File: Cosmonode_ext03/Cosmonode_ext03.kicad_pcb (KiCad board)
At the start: 2 copper layers, 23.5 x 34.3 mm, 8 parts, among them J1 CONN_01X04, J2 GS3, J3 GS3, J4 CONN_01X04, J5 CONN_01X08, J6 CONN_01X08, J7 Aloes_Logo, J8 OSHW_Logo

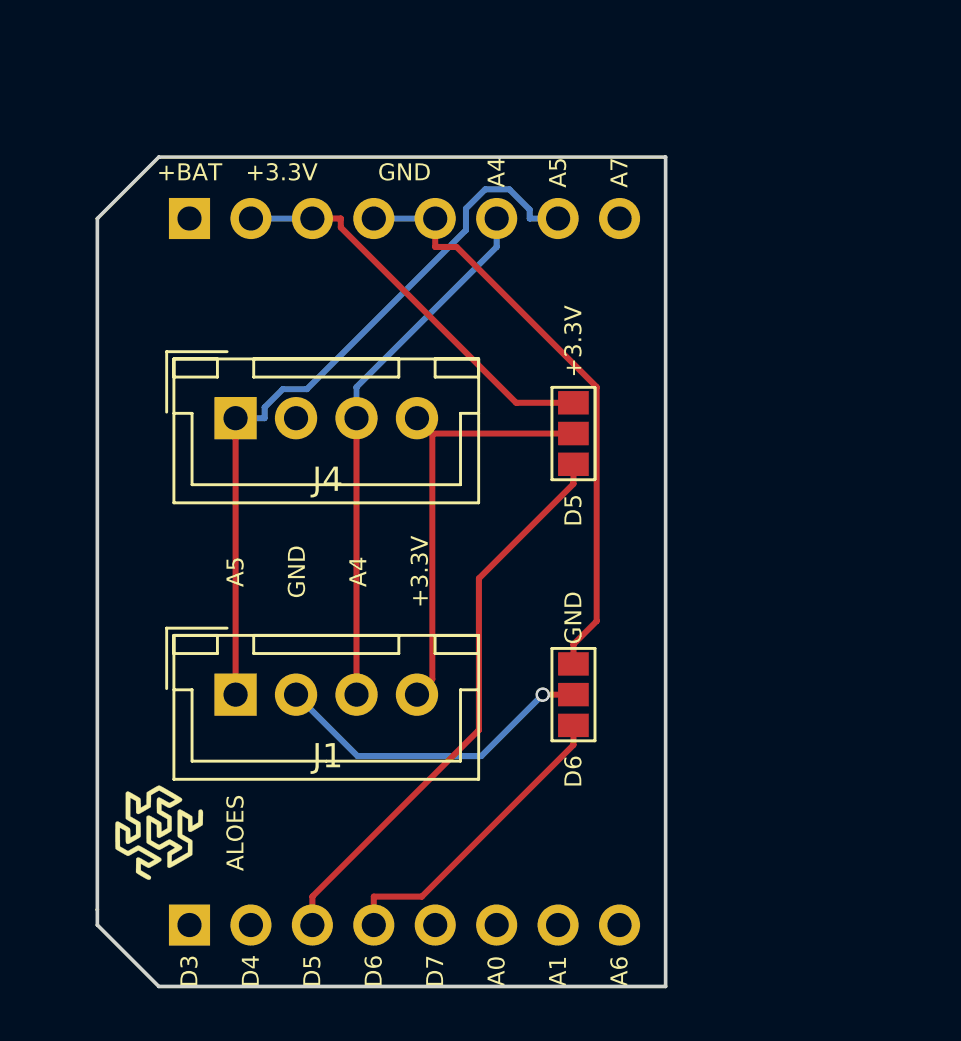
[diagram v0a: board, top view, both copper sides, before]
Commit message: update to V0.7 (WIP)
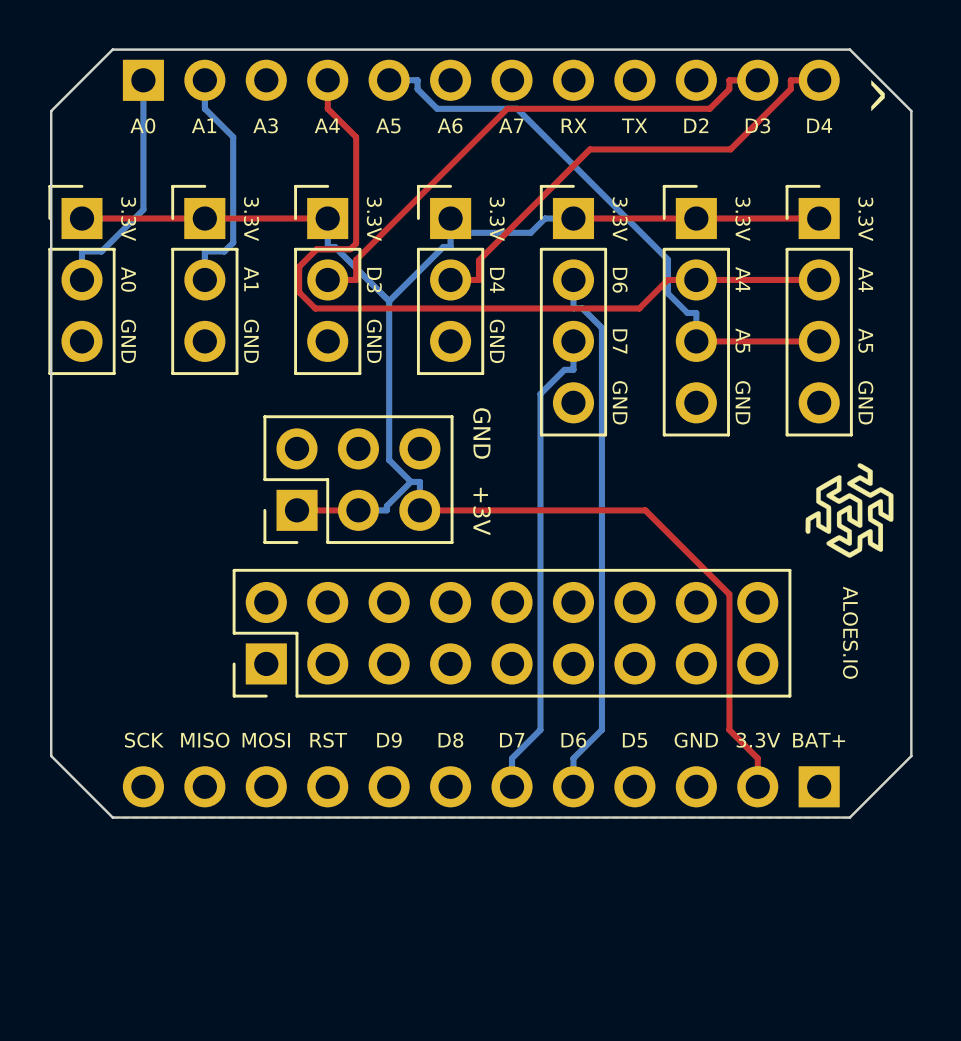
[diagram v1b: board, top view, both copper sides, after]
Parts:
- added J10: CONN_01X03, Pin_Headers:Pin_Header_Straight_1x03_Pitch2.54mm, F.Cu at (146.1, 97.2)
- added J11: CONN_01X03, Pin_Headers:Pin_Header_Straight_1x03_Pitch2.54mm, F.Cu at (151.1, 97.2)
- added J12: CONN_02X03, Pin_Headers:Pin_Header_Straight_2x03_Pitch2.54mm, F.Cu at (154.9, 109.2)
- added J13: CONN_02X09, Pin_Headers:Pin_Header_Straight_2x09_Pitch2.54mm, F.Cu at (153.7, 115.6)
- added J9: CONN_01X04, Pin_Headers:Pin_Header_Straight_1x04_Pitch2.54mm, F.Cu at (166.4, 97.2)
- J1: value CONN_01X04 -> OSHW_Logo; footprint Connectors_JST:JST_XH_B04B-XH-A_04x2.50mm_Straight -> Symbols:OSHW-Logo_5.7x6mm_SilkScreen; moved to B.Cu
- J2: value GS3 -> CONN_01X04; footprint Connectors:GS3 -> Pin_Headers:Pin_Header_Straight_1x04_Pitch2.54mm
- J3: value GS3 -> CONN_01X12; footprint Connectors:GS3 -> Socket_Strips:Socket_Strip_Straight_1x12_Pitch2.54mm; moved to B.Cu
- J4: value CONN_01X04 -> CONN_01X12; footprint Connectors_JST:JST_XH_B04B-XH-A_04x2.50mm_Straight -> Socket_Strips:Socket_Strip_Straight_1x12_Pitch2.54mm; moved to B.Cu
- J5, J6: value CONN_01X08 -> CONN_01X03; footprint Socket_Strips:Socket_Strip_Straight_1x08_Pitch2.54mm -> Pin_Headers:Pin_Header_Straight_1x03_Pitch2.54mm; moved to F.Cu
- J8: value OSHW_Logo -> CONN_01X04; footprint Symbols:OSHW-Logo_5.7x6mm_SilkScreen -> Pin_Headers:Pin_Header_Straight_1x04_Pitch2.54mm; moved to F.Cu
- moved J7 31.5 mm to (177.8, 109.2), turned to 270 degrees
- moved J5 31.1 mm to (161.3, 97.2), turned to 0 degrees
- moved J3 31.0 mm to (148.6, 91.4), turned to 270 degrees
- moved J4 28.5 mm to (176.5, 120.7), turned to 90 degrees
- moved J8 20.2 mm to (171.4, 97.2), turned to 0 degrees
- moved J2 13.5 mm to (176.5, 97.2), turned to 0 degrees
- moved J6 5.72 mm to (156.2, 97.2), turned to 0 degrees
- moved J1 4.58 mm to (148.6, 114.3), turned to 90 degrees
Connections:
- J2 pad 1: /D5 -> +3V3
- J2 pad 2: Net-(J1-Pad4) -> A4
- J2 pad 3: +3V3 -> A5
- J3 pad 1: /D6 -> A0
- J3 pad 2: Net-(J1-Pad2) -> A1
- J3 pad 3: GND -> A3
- J4 pad 1: /A5 -> +BATT
- J4 pad 2: Net-(J1-Pad2) -> +3V3
- J4 pad 3: /A4 -> GND
- J4 pad 4: Net-(J1-Pad4) -> D5
- J5 pad 1: /D3 -> +3V3
- J5 pad 2: /D4 -> D4
- J5 pad 3: /D5 -> GND
- J6 pad 1: /BAT+ -> +3V3
- J6 pad 2: +3V3 -> D3
- J6 pad 3: +3V3 -> GND
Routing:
- net +3V3: track 16.7 -> 72.3 mm
- net A4: track 0.00 -> 33.3 mm
- net /A5: track 30.2 -> 0.00 mm
- net GND: track 24.6 -> 0.00 mm
- net A5: track 0.00 -> 24.0 mm
- net /D5: track 23.5 -> 0.00 mm
- net D6: track 0.00 -> 22.1 mm
- net /A4: track 22.1 -> 0.00 mm
- net D3: track 0.00 -> 21.9 mm
- net D7: track 0.00 -> 19.7 mm
- net D4: track 0.00 -> 19.3 mm
- net Net-(J1-Pad4): track 17.8 -> 0.00 mm
- net Net-(J1-Pad2): track 13.6 -> 0.00 mm, vias 1 -> 0
- net /D6: track 12.8 -> 0.00 mm
- net A0: track 0.00 -> 9.78 mm
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- added copper zone on B.Cu, net GND
- added copper zone on F.Cu, net GND
- removed copper zone on F.Cu, net Net-(J1-Pad2)
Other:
- board size 23.5 x 34.3 mm -> 35.6 x 31.8 mm
- rule pad_to_mask_clearance: 0.2 -> 0
- board text added: "+3V"
- board text added: "3.3V"
- board text added: "A3"
- board text added: "ALOES.IO"
- board text added: "BAT+"
- board text added: "D2"
- board text added: "D8"
- board text added: "D9"
- board text added: "Extension #3 ProtoBoard"
- board text added: "MISO"
- board text added: "MOSI"
- board text added: "RST"
- board text added: "RX"
- board text added: "SCK"
- board text added: "TX"
- board text added: "^"
- board text removed: "+3.3V"
- board text removed: "+BAT"
- board text removed: "ALOES"
- board text removed: "Extension #2 I2C connectors"
